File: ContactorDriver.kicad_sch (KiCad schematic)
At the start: 43 parts, among them J1 PowerConn, J10 FanConn3, J11 FanConn4, J2 DashboardConnA, J3 ContactorAConn, J4 DashboardConnB, J5 ContactorBConn, J6 DashboardConnC, J7 ContactorCConn, J8 FanConn1, J9 FanConn2, Q1 PMV35EPER, Q2 IRLML0030TRPbF, Q3 IRLML0030TRPbF, Q4 IRLML0030TRPbF

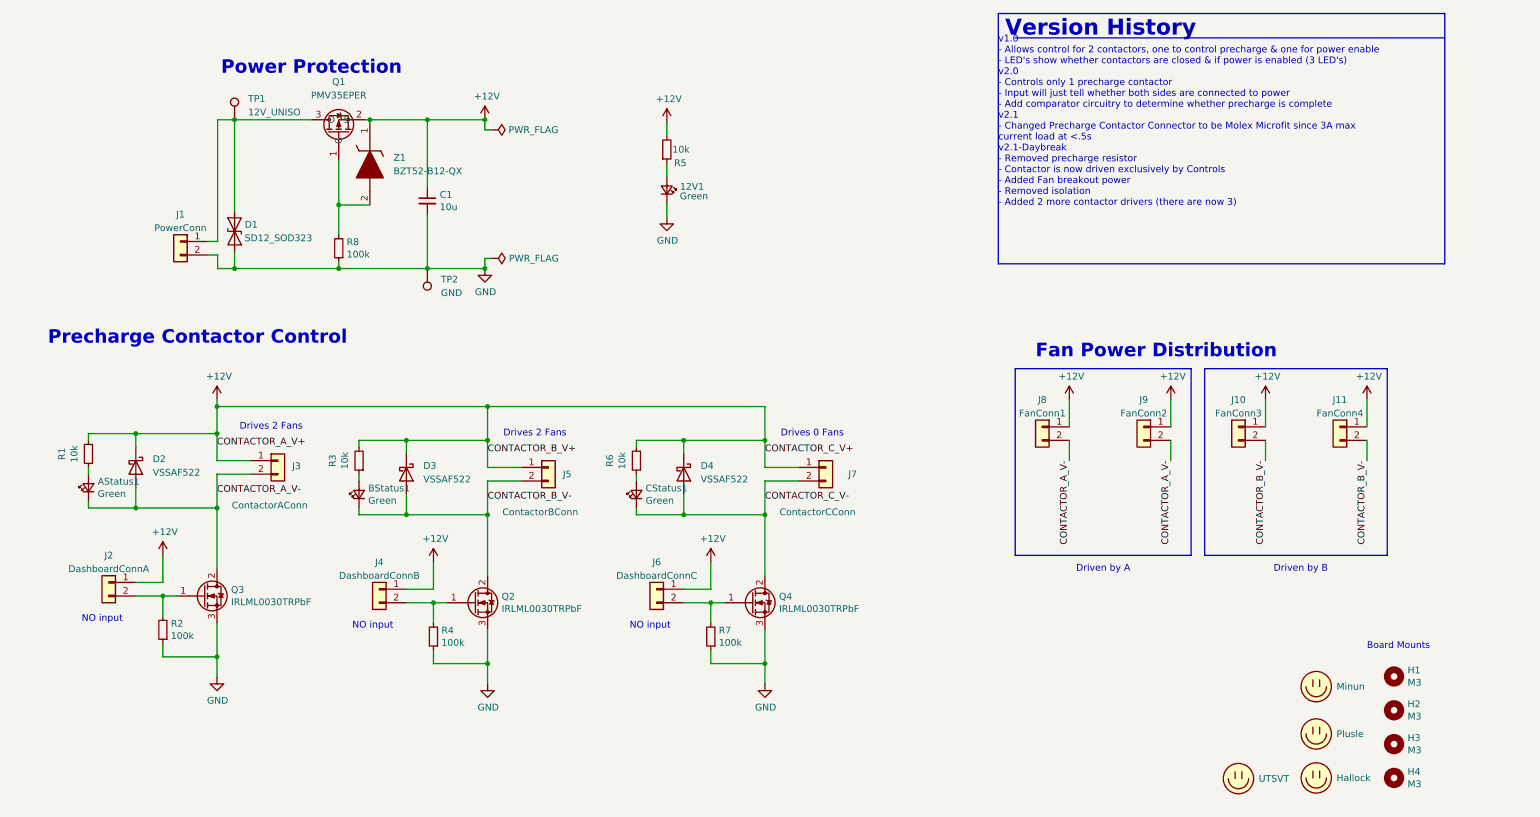
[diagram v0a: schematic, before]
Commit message: added sense
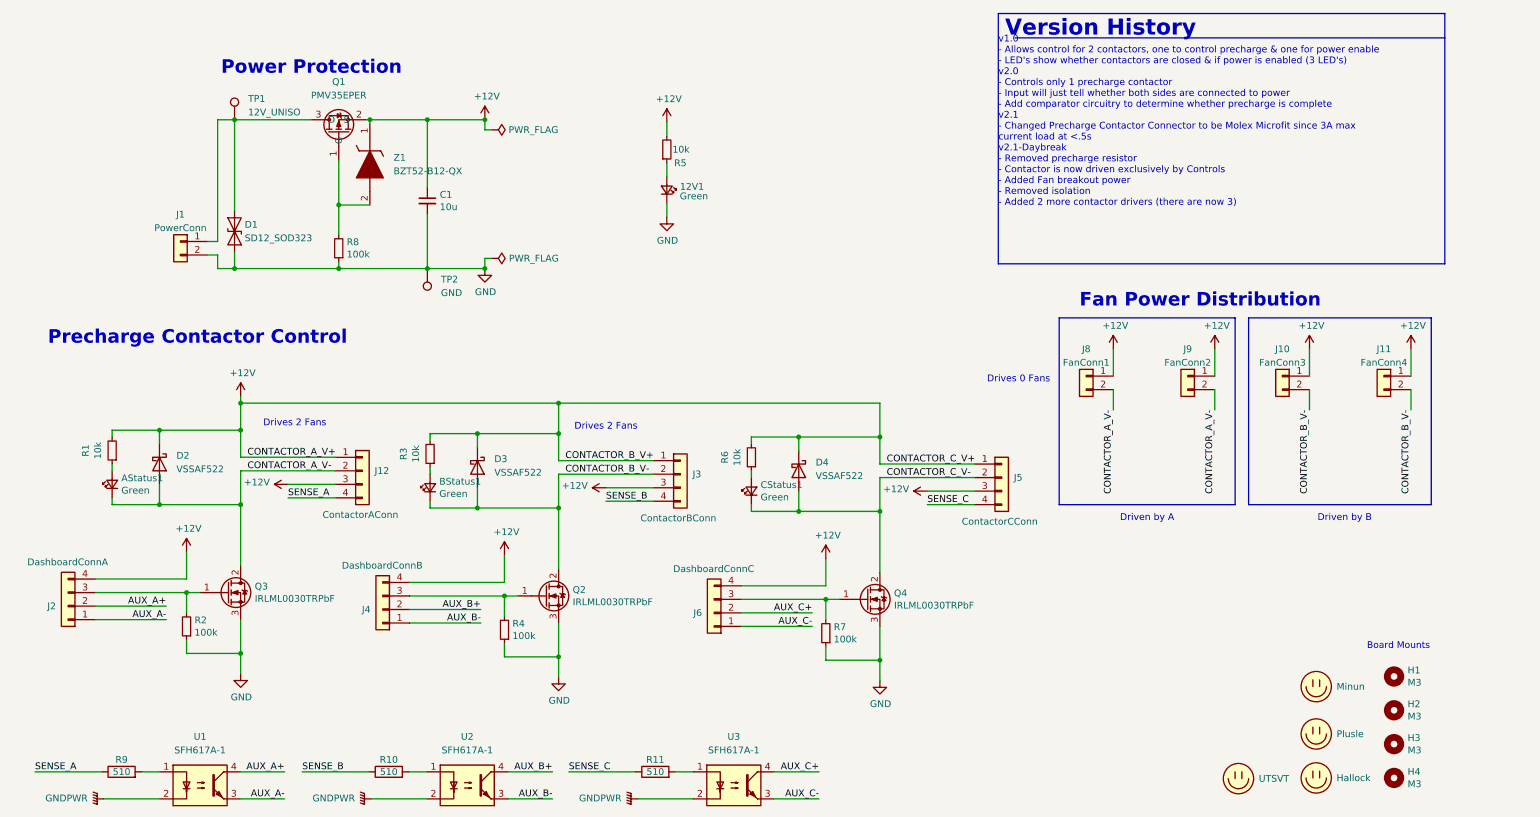
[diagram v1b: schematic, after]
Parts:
- removed J2: DashboardConnA, Connector_Molex:Molex_Micro-Fit_3.0_43650-0215_1x02_P3.00mm_Vertical, symbol Connector_Generic:Conn_01x02
- removed J3: ContactorAConn, Connector_Molex:Molex_Micro-Fit_3.0_43650-0215_1x02_P3.00mm_Vertical, symbol Connector_Generic:Conn_01x02
- removed J4: DashboardConnB, Connector_Molex:Molex_Micro-Fit_3.0_43650-0215_1x02_P3.00mm_Vertical, symbol Connector_Generic:Conn_01x02
- removed J5: ContactorBConn, Connector_Molex:Molex_Micro-Fit_3.0_43650-0215_1x02_P3.00mm_Vertical, symbol Connector_Generic:Conn_01x02
- removed J6: DashboardConnC, Connector_Molex:Molex_Micro-Fit_3.0_43650-0215_1x02_P3.00mm_Vertical, symbol Connector_Generic:Conn_01x02
- removed J7: ContactorCConn, Connector_Molex:Molex_Micro-Fit_3.0_43650-0215_1x02_P3.00mm_Vertical, symbol Connector_Generic:Conn_01x02
- added J12: ContactorAConn, UTSVT_Connectors:Molex_MicroFit3.0_1x4xP3.00mm_PolarizingPeg_Vertical, symbol Connector_Generic:Conn_01x04
- added J2: DashboardConnA, UTSVT_Connectors:Molex_MicroFit3.0_1x4xP3.00mm_PolarizingPeg_Vertical, symbol Connector_Generic:Conn_01x04
- added J3: ContactorBConn, UTSVT_Connectors:Molex_MicroFit3.0_1x4xP3.00mm_PolarizingPeg_Vertical, symbol Connector_Generic:Conn_01x04
- added J4: DashboardConnB, UTSVT_Connectors:Molex_MicroFit3.0_1x4xP3.00mm_PolarizingPeg_Vertical, symbol Connector_Generic:Conn_01x04
- added J5: ContactorCConn, UTSVT_Connectors:Molex_MicroFit3.0_1x4xP3.00mm_PolarizingPeg_Vertical, symbol Connector_Generic:Conn_01x04
- added J6: DashboardConnC, UTSVT_Connectors:Molex_MicroFit3.0_1x4xP3.00mm_PolarizingPeg_Vertical, symbol Connector_Generic:Conn_01x04
- added R10, R11, R9: 510, Resistor_SMD:R_0805_2012Metric_Pad1.20x1.40mm_HandSolder, symbol Device:R
- added U1, U2, U3: SFH617A-1, Package_DIP:DIP-4_W7.62mm, symbol Isolator:SFH617A-1
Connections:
- net +12V: now also J12.1 (Pin_1), J12.3 (Pin_3), J2.4 (Pin_4), J3.1 (Pin_1), J3.3 (Pin_3), J4.4 (Pin_4), J5.1 (Pin_1), J5.3 (Pin_3), J6.4 (Pin_4)
- net CONTACTOR_A_V-: now also J12.2 (Pin_2)
- net CONTACTOR_B_V-: now also J3.2 (Pin_2)
- net CONTACTOR_C_V-: now also J5.2 (Pin_2)
- net at Q3.1 (G), R2.2: now also J2.3 (Pin_3)
- net at Q4.1 (G), R7.2: now also J6.3 (Pin_3)
- net at Q2.1 (G), R4.2: now also J4.3 (Pin_3)
- new net: R10.2, U2.1
- new net: R9.2, U1.1
- new net: R11.2, U3.1
- new net AUX_A+: J2.2 (Pin_2), U1.4
- new net AUX_A-: J2.1 (Pin_1), U1.3
- new net AUX_B+: J4.2 (Pin_2), U2.4
- new net AUX_B-: J4.1 (Pin_1), U2.3
- new net AUX_C+: J6.2 (Pin_2), U3.4
- new net AUX_C-: J6.1 (Pin_1), U3.3
- new net GNDPWR: U1.2, U2.2, U3.2
- new net SENSE_A: J12.4 (Pin_4), R9.1
- new net SENSE_B: J3.4 (Pin_4), R10.1
- new net SENSE_C: J5.4 (Pin_4), R11.1
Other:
- note removed: "NO input"
- moved on the sheet: AStatus1, BStatus1, CStatus1, D2, D3, D4, J10, J11, J8, J9, Q2, Q3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
